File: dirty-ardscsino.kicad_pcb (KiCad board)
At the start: 2 copper layers, 42.7 x 75.2 mm, 16 parts, among them J1 SCSI, J2 171825-4 (Ext. Power), J3 DM3AT-SF-PEJM5, U1 STM32 Bluepill

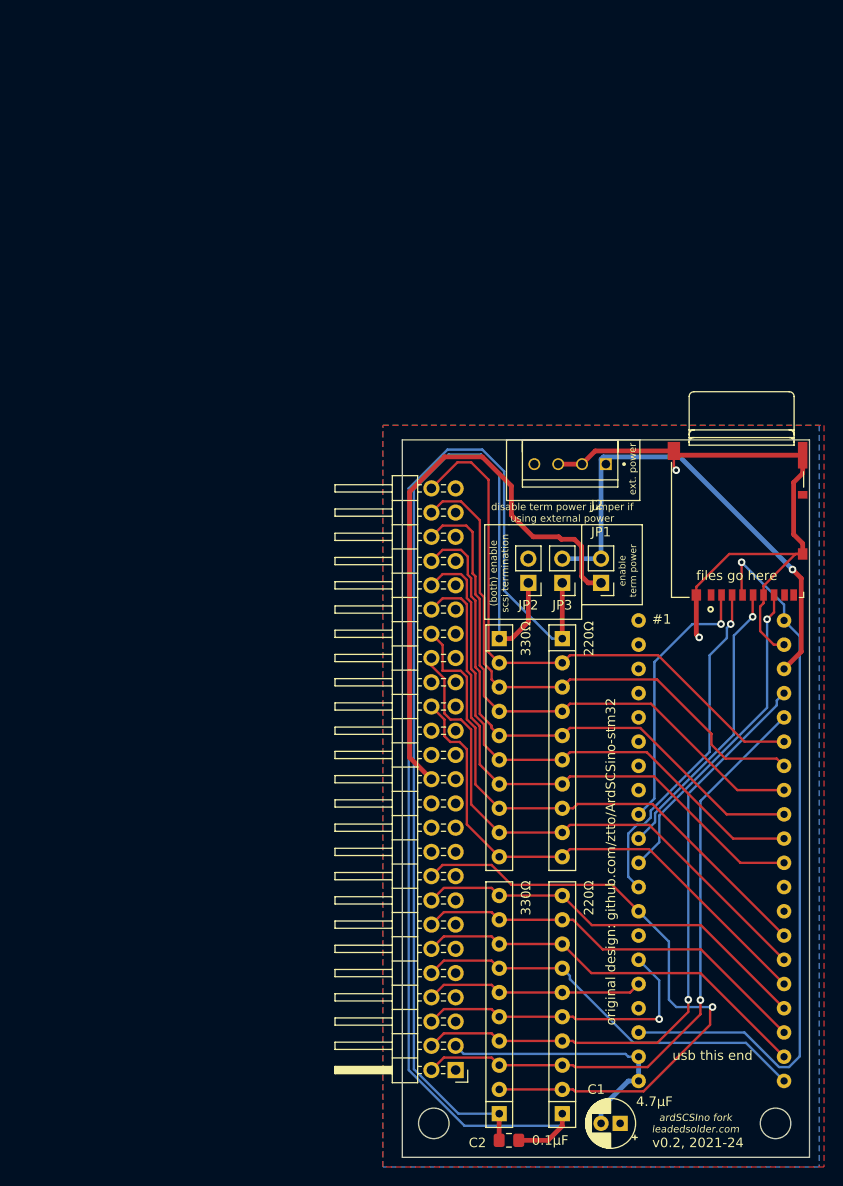
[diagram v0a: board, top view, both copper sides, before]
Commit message: Dirty ArdSCSIno 2 v1 sent to fab
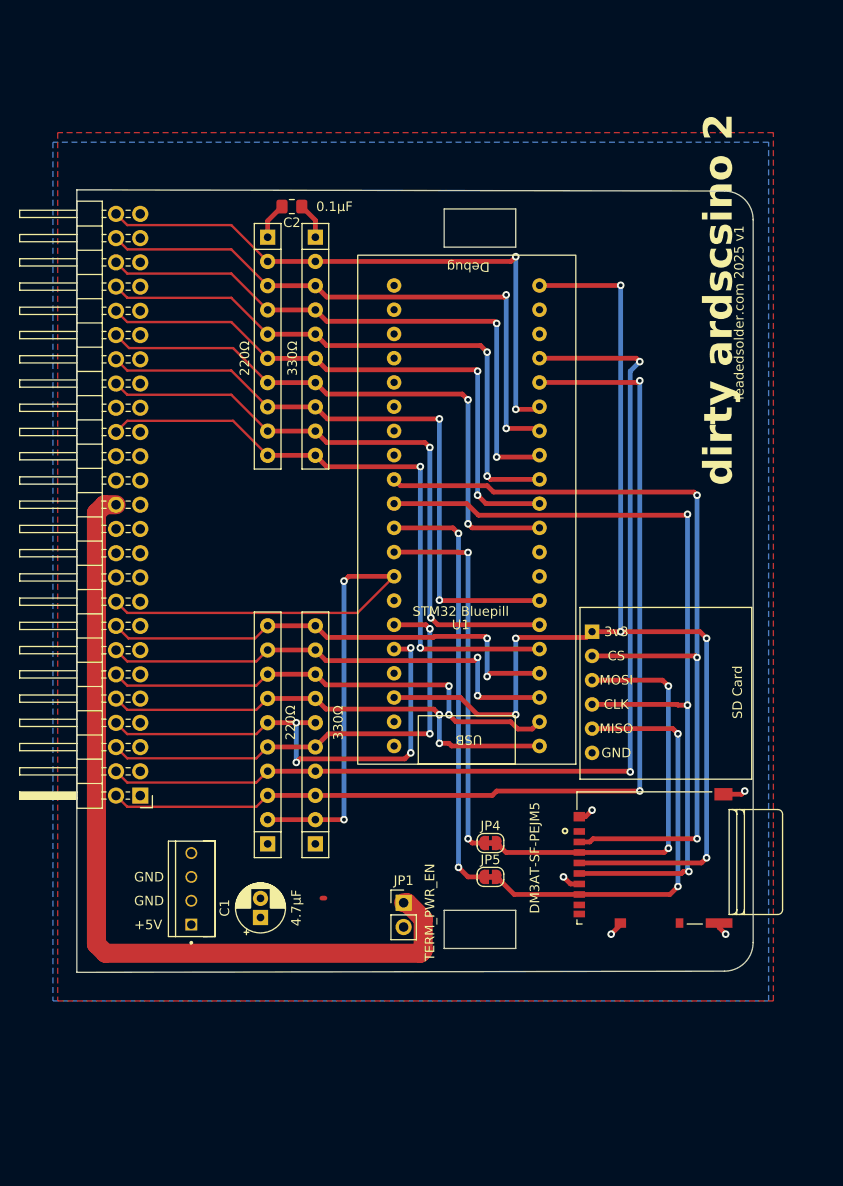
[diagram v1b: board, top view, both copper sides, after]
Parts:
- removed JP2, JP3: Jumper_NC_Small, Connector_PinHeader_2.54mm:PinHeader_1x02_P2.54mm_Vertical
- removed REF** (x2): MountingHole_3.2mm_M3, MountingHole:MountingHole_3.2mm_M3
- removed REF**: OSHW-Logo2_14.6x12mm_SilkScreen, Symbol:OSHW-Logo2_14.6x12mm_SilkScreen
- added JP4: Jumper_2_Small_Bridged, Jumper:SolderJumper-2_P1.3mm_Bridged_RoundedPad1.0x1.5mm, F.Cu at (143.3, 118.5)
- added JP5: Jumper_2_Small_Bridged, Jumper:SolderJumper-2_P1.3mm_Bridged_RoundedPad1.0x1.5mm, F.Cu at (143.3, 122.0)
- added U2: microSD-Breakout, microSD_Breakout:microSD_AliExpress, F.Cu at (152.7, 93.8)
- C2: footprint Capacitor_SMD:C_0805_2012Metric_Pad1.15x1.40mm_HandSolder -> Capacitor_SMD:C_0805_2012Metric_Pad1.18x1.45mm_HandSolder
- JP1: value Jumper_NC_Small -> TERM_PWR_EN
- moved C2 100.5 mm to (122.5, 51.8), turned to 180 degrees
- moved J2 64.9 mm to (112.0, 127.0), turned to 90 degrees
- moved RN1 52.2 mm to (120.0, 55.0)
- moved RN2 46.3 mm to (125.0, 55.0)
- moved J1 43.8 mm to (106.7, 113.5)
- moved U1 43.5 mm to (139.0, 87.3)
- moved C1 43.4 mm to (119.2, 126.2), turned to 90 degrees
- moved RN4 41.9 mm to (120.0, 118.5)
- moved JP1 39.4 mm to (134.2, 124.7), turned to 0 degrees
- moved RN3 34.2 mm to (125.0, 118.5)
- moved J3 32.7 mm to (152.7, 120.4), turned to 90 degrees
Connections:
- C2 pad 1: Net-(C2-Pad1) -> GND
- C2 pad 2: Net-(C2-Pad2) -> +5V
- J1 pad 25: Net-(J1-Pad25) -> unconnected-(J1-Pin_25-Pad25)
- J2 pad 4: Net-(J2-Pad4) -> unconnected-(J2-Pad4)
- J3 pad 1: Net-(J3-Pad1) -> unconnected-(J3-DAT2-Pad1)
- J3 pad 8: Net-(J3-Pad8) -> unconnected-(J3-DAT1-Pad8)
- J3 pad SWA: Net-(J3-PadSWA) -> unconnected-(J3-PadSWA)
- J3 pad SWB: Net-(J3-PadSWB) -> unconnected-(J3-PadSWB)
- RN1 pad 1: Net-(C2-Pad2) -> +5V
- RN2 pad 1: Net-(C2-Pad1) -> GND
- RN3 pad 1: Net-(C2-Pad1) -> GND
- RN4 pad 1: Net-(C2-Pad2) -> +5V
- U1 pad NRST: Net-(U1-PadNRST) -> unconnected-(U1-RESET-PadNRST)
- U1 pad PA0: Net-(U1-PadPA0) -> unconnected-(U1-PadPA0)
- U1 pad PA1: Net-(U1-PadPA1) -> unconnected-(U1-PadPA1)
- U1 pad PA11: Net-(U1-PadPA11) -> unconnected-(U1-PadPA11)
- U1 pad PA12: Net-(U1-PadPA12) -> unconnected-(U1-PadPA12)
- U1 pad PA2: Net-(U1-PadPA2) -> unconnected-(U1-PadPA2)
- U1 pad PA3: Net-(U1-PadPA3) -> unconnected-(U1-PadPA3)
- U1 pad PA6: /SD_MISO -> /BP_MISO
- U1 pad PA7: /SD_MOSI -> /BP_MOSI
- U1 pad PB1: Net-(U1-PadPB1) -> unconnected-(U1-PadPB1)
- U1 pad PC13: Net-(U1-PadPC13) -> unconnected-(U1-PadPC13)
- U1 pad PC14: Net-(U1-PadPC14) -> unconnected-(U1-PadPC14)
- U1 pad PC15: Net-(U1-PadPC15) -> unconnected-(U1-PadPC15)
- U1 pad VBAT: Net-(U1-PadVBAT) -> unconnected-(U1-Vbat-PadVBAT)
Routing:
- net Net-(C2-Pad2): track 126.2 -> 0.00 mm
- net Net-(C2-Pad1): track 111.0 -> 0.00 mm
- net GND: track 99.5 -> 12.8 mm, vias 2 -> 5
- net /SD_CS: track 28.4 -> 92.0 mm, vias 1 -> 3
- net /SD_CSK: track 30.5 -> 90.4 mm, vias 1 -> 3
- net +5V: track 51.1 -> 4.15 mm, vias 1 -> 0
- net /SD_VCC: track 76.6 -> 123.5 mm, vias 1 -> 6
- net /BP_MISO: track 0.00 -> 45.1 mm, vias 0 -> 2
- net /SCSI_DAT0: track 66.2 -> 109.6 mm, vias 1 -> 2
- net /SCSI_DAT1: track 66.8 -> 109.0 mm, vias 1 -> 2
- net /BP_MOSI: track 0.00 -> 39.7 mm, vias 0 -> 2
- net /SCSI_DAT3: track 23.0 -> 51.2 mm, vias 0 -> 4
- net /TERM_POWER: track 61.7 -> 88.4 mm
- net /SCSI_DAT2: track 32.0 -> 49.4 mm, vias 1 -> 2
- net /SD_MISO: track 34.1 -> 45.3 mm, vias 1 -> 2
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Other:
- board size 42.7 x 75.2 mm -> 70.9 x 82 mm
- rule pad_to_mask_clearance: 0.051 -> 0
- board text added: "dirty ardscsino 2"
- board text added: "leadedsolder.com 2025 v1"
- board text removed: "#1"
- board text removed: "(both) enable scsi termination"
- board text removed: "220Ω"
- board text removed: "330Ω"
- board text removed: "3v3"
- board text removed: "5v"
- board text removed: "ACK"
- board text removed: "ATN"
- board text removed: "Busy"
- board text removed: "CD"
- board text removed: "DBP"
- board text removed: "Data 0"
- board text removed: "Data 1"
- board text removed: "Data 2"
- board text removed: "Data 3"
- board text removed: "Data 4"
- board text removed: "Data 5"
- board text removed: "Data 6"
- board text removed: "Data 7"
- board text removed: "I/O"
- board text removed: "MSG"
- board text removed: "REQ"
- board text removed: "Reset"
- board text removed: "SEL"
- board text removed: "Term. Power"
- board text removed: "ardSCSIno fork leadedsolder.com"
- board text removed: "disable term power jumper if using external power"
- board text removed: "enable term power"
- board text removed: "ext. power"
- board text removed: "files go here"
- board text removed: "original design: github.com/ztto/ArdSCSino-stm32"
- board text removed: "usb this end"
- board text removed: "v0.2, 2021-24"
